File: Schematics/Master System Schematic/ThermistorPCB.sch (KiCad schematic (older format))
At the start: 28 parts

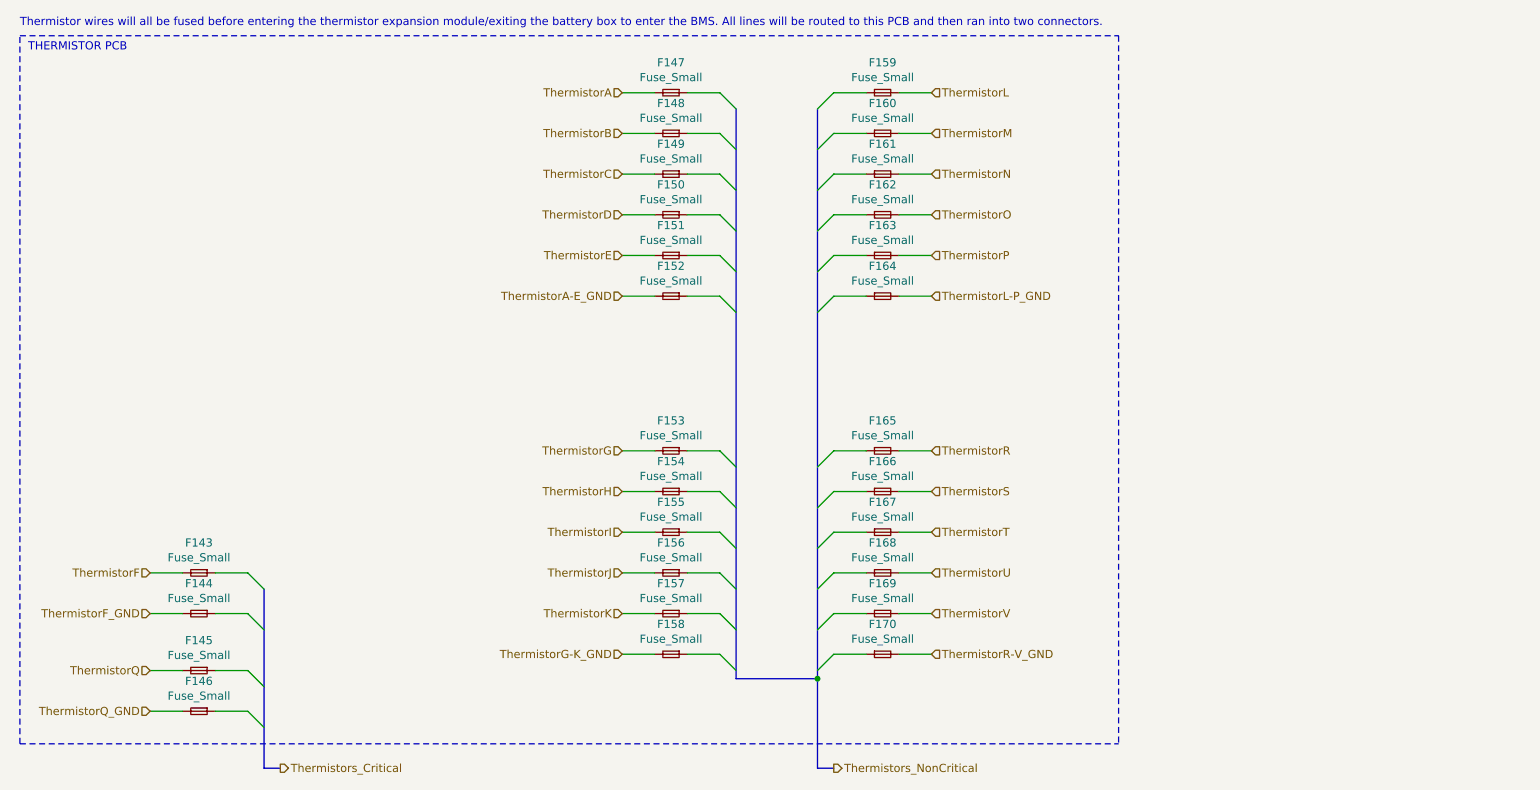
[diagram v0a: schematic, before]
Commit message: fixed therm boards
fixed therm board implementation
beginning accumulator redraw
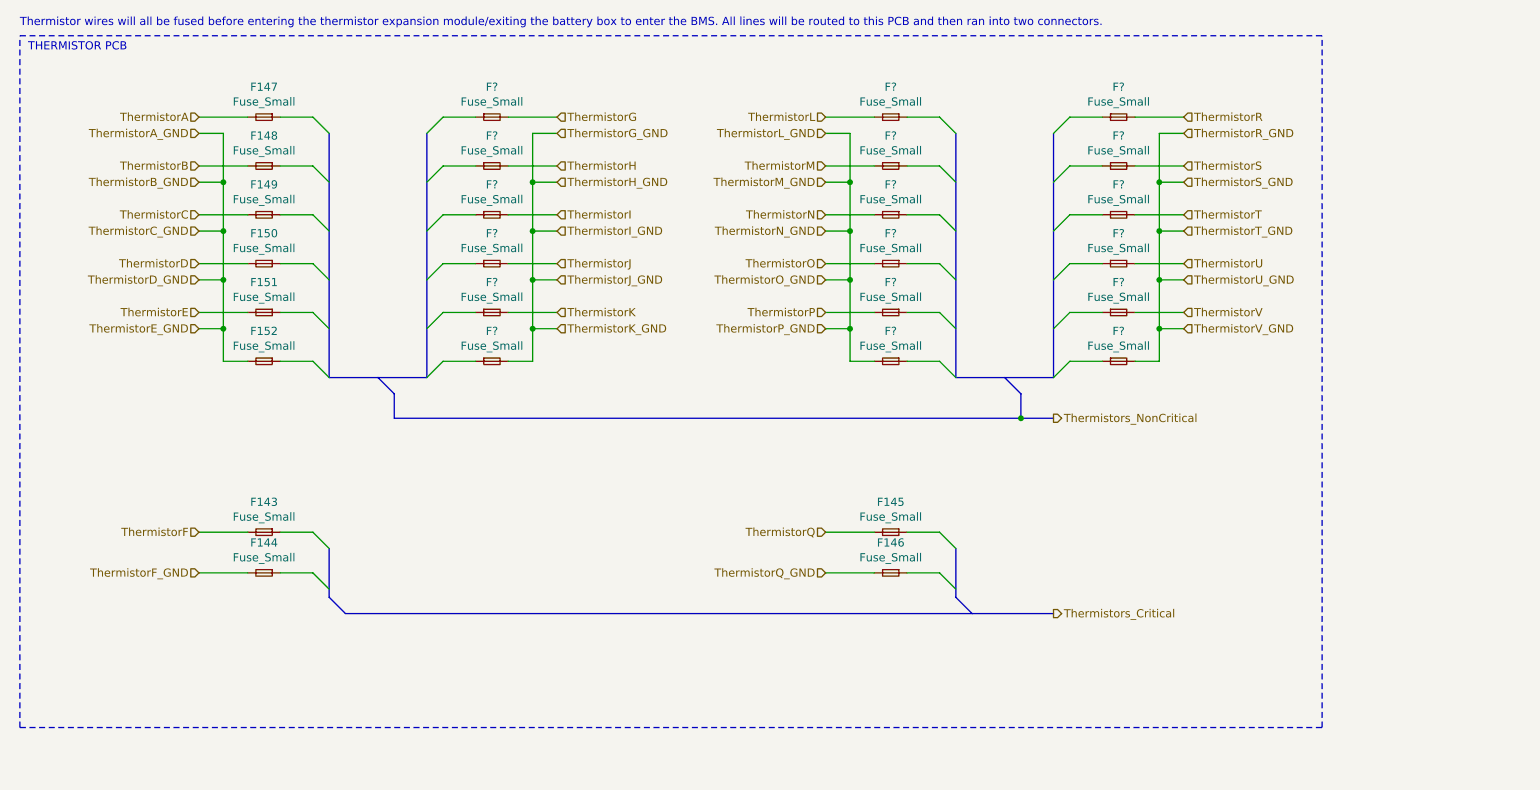
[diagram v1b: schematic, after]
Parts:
- removed F153, F154, F155, F156, F157, F158, F159, F160, F161, F162, F163, F164, F165, F166, F167, F168, F169, F170: Fuse_Small, symbol Device:Fuse_Small
- added F? (x18): Fuse_Small, symbol Device:Fuse_Small
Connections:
- net ThermistorG: now also F?.2
- net ThermistorH: now also F?.2
- net ThermistorI: now also F?.2
- net ThermistorJ: now also F?.2
- net ThermistorK: now also F?.2
- net ThermistorL: now also F?.2
- net ThermistorM: now also F?.2
- net ThermistorN: now also F?.2
- net ThermistorO: now also F?.2
- net ThermistorP: now also F?.2
- net ThermistorR: now also F?.2
- net ThermistorS: now also F?.2
- net ThermistorT: now also F?.2
- net ThermistorU: now also F?.2
- net ThermistorV: now also F?.2
- net ThermistorA-E_GND renamed ThermistorA_GND
- new net ThermistorG_GND: F?.2
- new net ThermistorL_GND: F?.2
- new net ThermistorR_GND: F?.2
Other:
- moved on the sheet: F143, F144, F145, F146, F147, F148, F149, F150, F151, F152
